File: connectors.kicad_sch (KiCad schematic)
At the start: 3 parts, among them J1 112-024-113R001, J3 RJHSE5380, J4 USB4085-GF-A

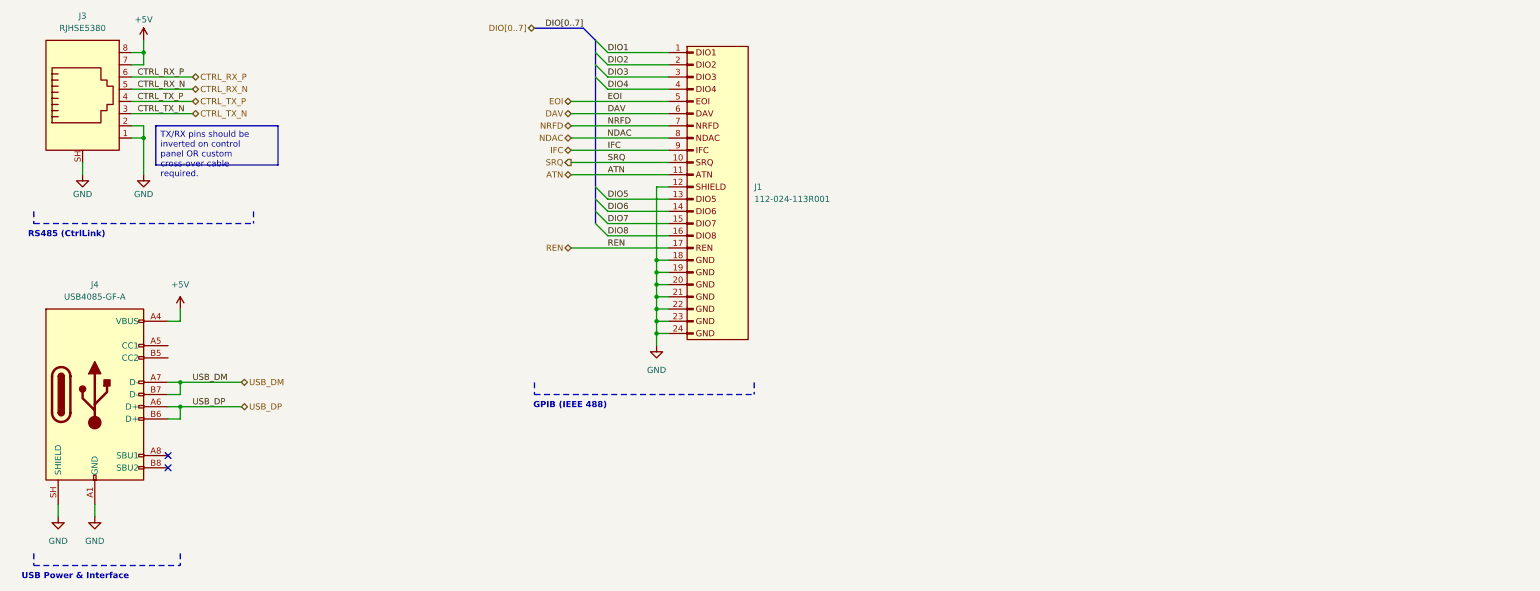
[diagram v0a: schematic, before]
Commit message: Finish up schematics
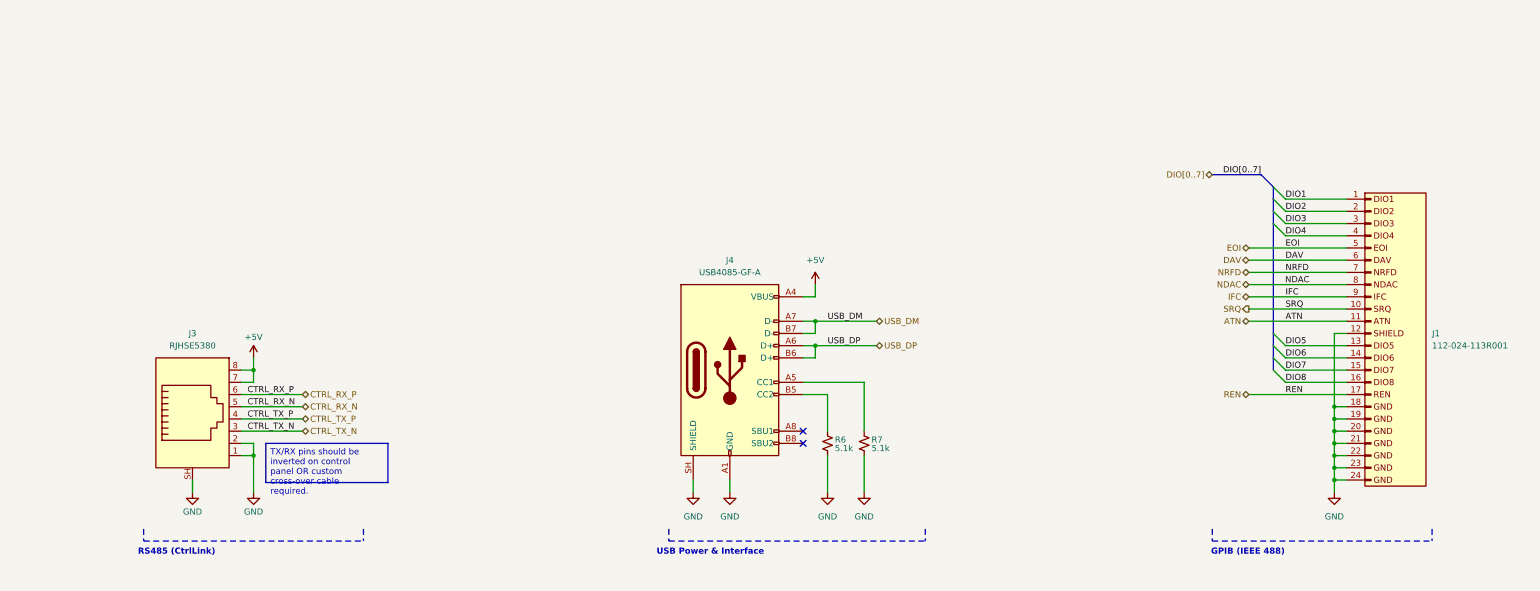
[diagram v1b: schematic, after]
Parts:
- added R6, R7: 5.1k, Resistor_SMD:R_0603_1608Metric, symbol PARTSDB:RC0603FR-075K1L
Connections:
- net DIO5: now also J1.13 (Pin_13)
- net GND: now also R6.2, R7.2
- net at J4.A5 (CC1): now also R7.1
- net at J4.B5 (CC2): now also R6.1
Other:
- title: (none) -> Connectors
- moved on the sheet: J1, J3, J4
